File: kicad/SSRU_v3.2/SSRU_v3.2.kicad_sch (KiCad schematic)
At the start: 68 parts, among them J2 Conn_01x24, J31 Conn_01x04, J4 AVR-ISP-6, J5 Conn_01x03, SW1 SW_Push, U1 MCP2515-xST, U10 TJA1051T, U12 TJA1051T, U2 ATmega328P-A, U3 LM2904, U4 LM2576S-5, U6 MCP2515-xST, U8 74LVC1G17, Y1 16MHz, Y3 20MHz, Y4 20MHz

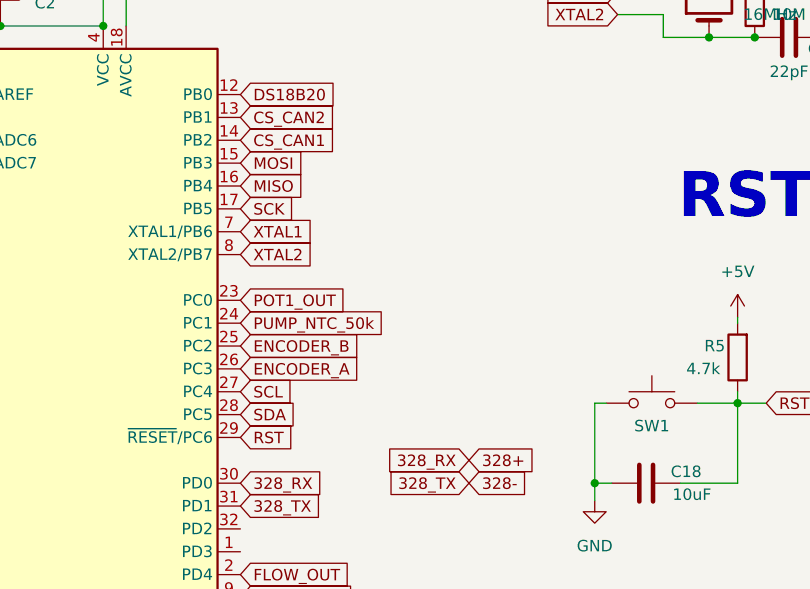
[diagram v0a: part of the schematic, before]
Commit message: gerbers
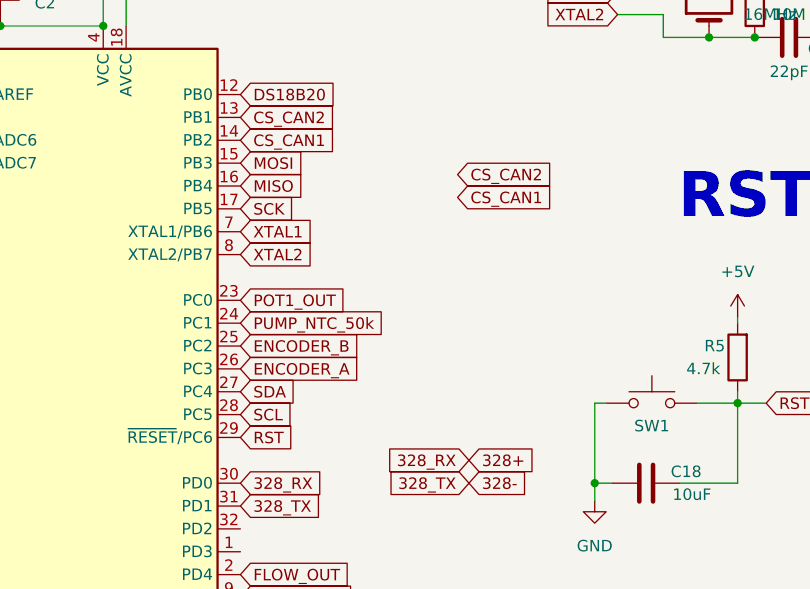
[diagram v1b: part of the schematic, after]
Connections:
- net I2C+: now also U2.28 (PC5); no longer U2.27 (PC4)
- net I2C-: now also U2.27 (PC4); no longer U2.28 (PC5)
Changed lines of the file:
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@@
 	(global_label "SCL"
 		(shape input)
-		(at 92.71 67.31 0)
-		(fields_autoplaced yes)
-		(effects
-			(font
-				(size 1.27 1.27)
-			)
-			(justify left)
-		)
-		(property "Intersheetrefs" "${INTERSHEET_REFS}"
-			(at 99.2028 67.31 0)
+		(at 92.71 69.85 0)
+		(fields_autoplaced yes)
+		(effects
+			(font
+				(size 1.27 1.27)
+			)
+			(justify left)
+		)
+		(property "Intersheetrefs" "${INTERSHEET_REFS}"
+			(at 99.2633 69.85 0)
 			(effects
 				(font
@@
 		)
 	)
+	(global_label "CS_CAN2"
+		(shape input)
+		(at 116.84 43.18 0)
+		(fields_autoplaced yes)
+		(effects
+			(font
+				(size 1.27 1.27)
+			)
+			(justify left)
+		)
+		(property "Intersheetrefs" "${INTERSHEET_REFS}"
+			(at 129.0175 43.18 0)
+			(effects
+				(font
+					(size 1.27 1.27)
+				)
+				(justify left)
+				(hide yes)
+			)
+		)
+	)
 	(global_label "POT1_IN"
 		(shape input)
@@
 				)
 				(justify right)
+				(hide yes)
+			)
+		)
+	)
+	(global_label "CS_CAN1"
+		(shape input)
+		(at 116.84 45.72 0)
+		(fields_autoplaced yes)
+		(effects
+			(font
+				(size 1.27 1.27)
+			)
+			(justify left)
+		)
+		(property "Intersheetrefs" "${INTERSHEET_REFS}"
+			(at 128.1709 45.72 0)
+			(effects
+				(font
+					(size 1.27 1.27)
+				)
+				(justify left)
 				(hide yes)
 			)
@@
 	(global_label "SDA"
 		(shape input)
-		(at 92.71 69.85 0)
-		(fields_autoplaced yes)
-		(effects
-			(font
-				(size 1.27 1.27)
-			)
-			(justify left)
-		)
-		(property "Intersheetrefs" "${INTERSHEET_REFS}"
-			(at 99.2633 69.85 0)
-			(effects
-				(font
+		(at 92.71 67.31 0)
+		(fields_autoplaced yes)
+		(effects
+			(font
+				(size 1.27 1.27)
+			)
+			(justify left)
+		)
+		(property "Intersheetrefs" "${INTERSHEET_REFS}"
+			(at 99.2028 67.31 0)
+			(effects
+				(font
